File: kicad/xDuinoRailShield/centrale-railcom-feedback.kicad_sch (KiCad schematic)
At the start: 0 parts

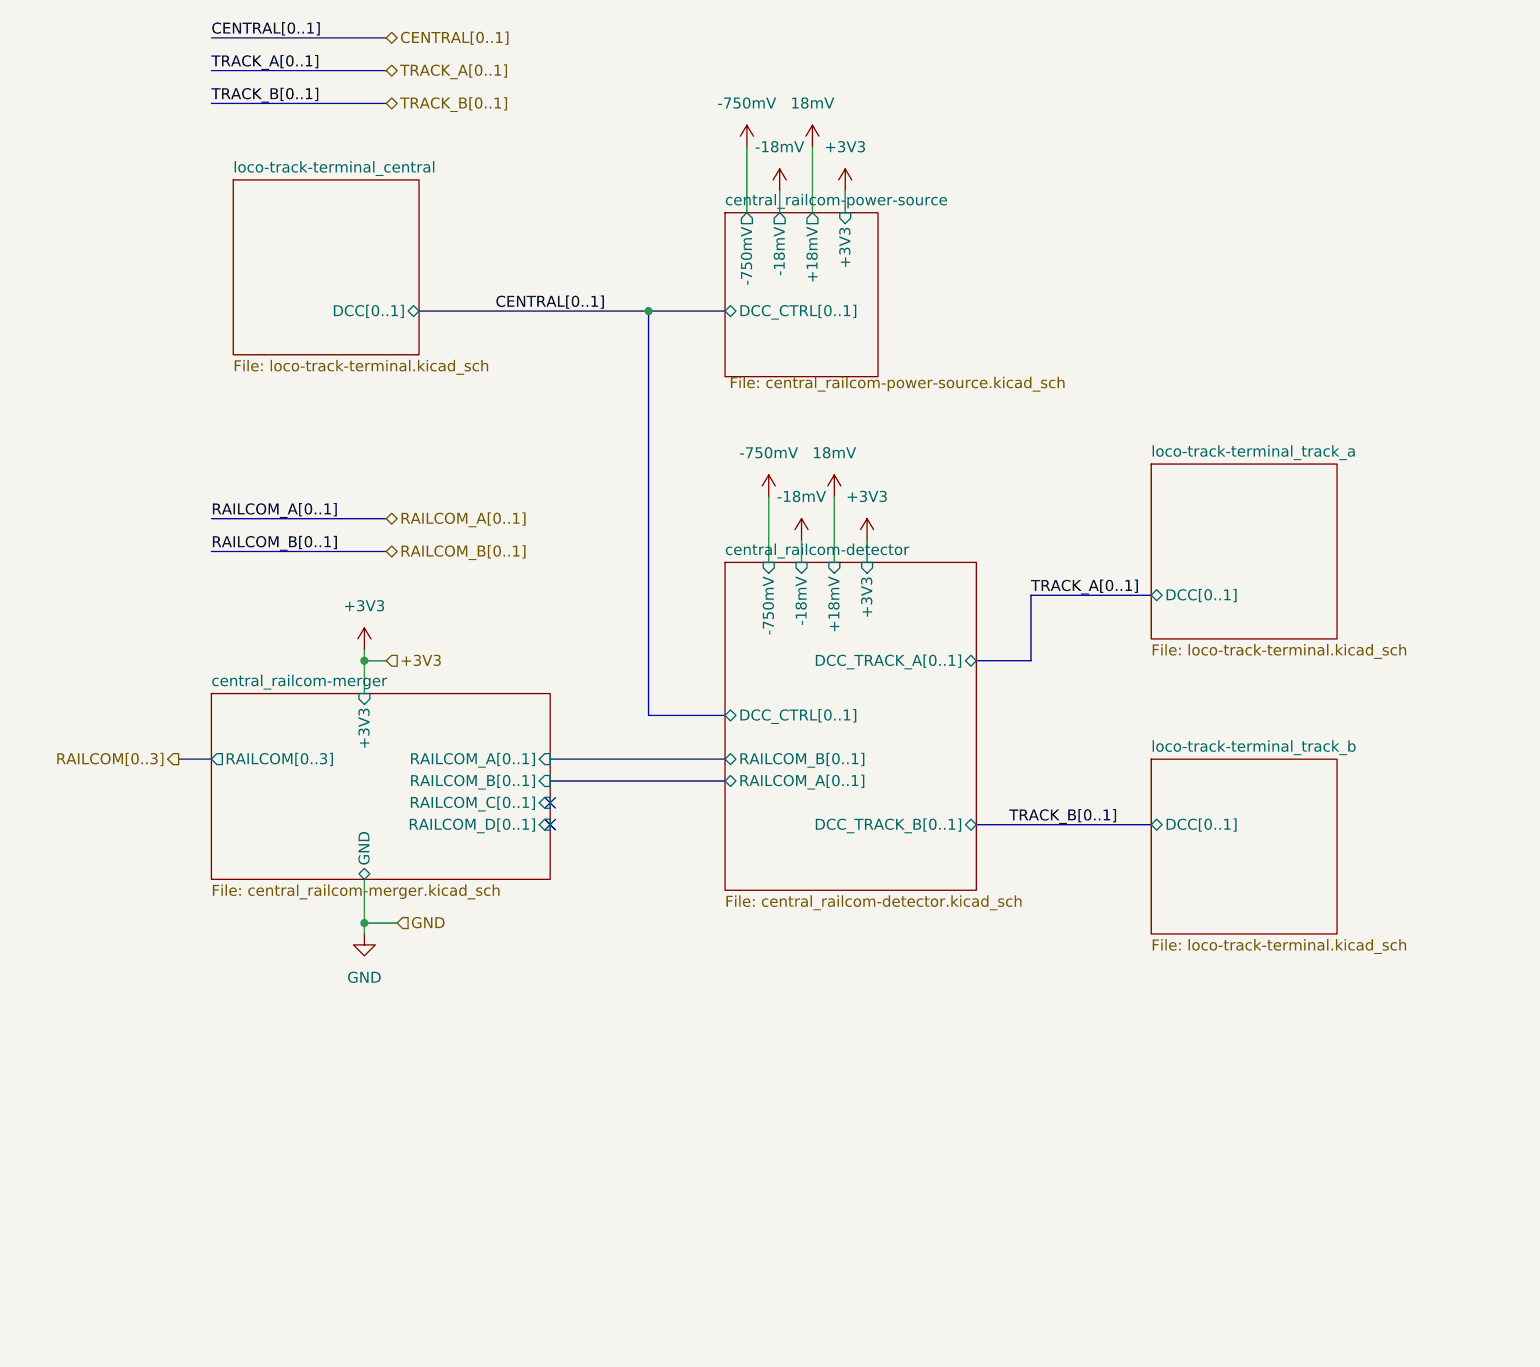
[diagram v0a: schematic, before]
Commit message: Many exiting news
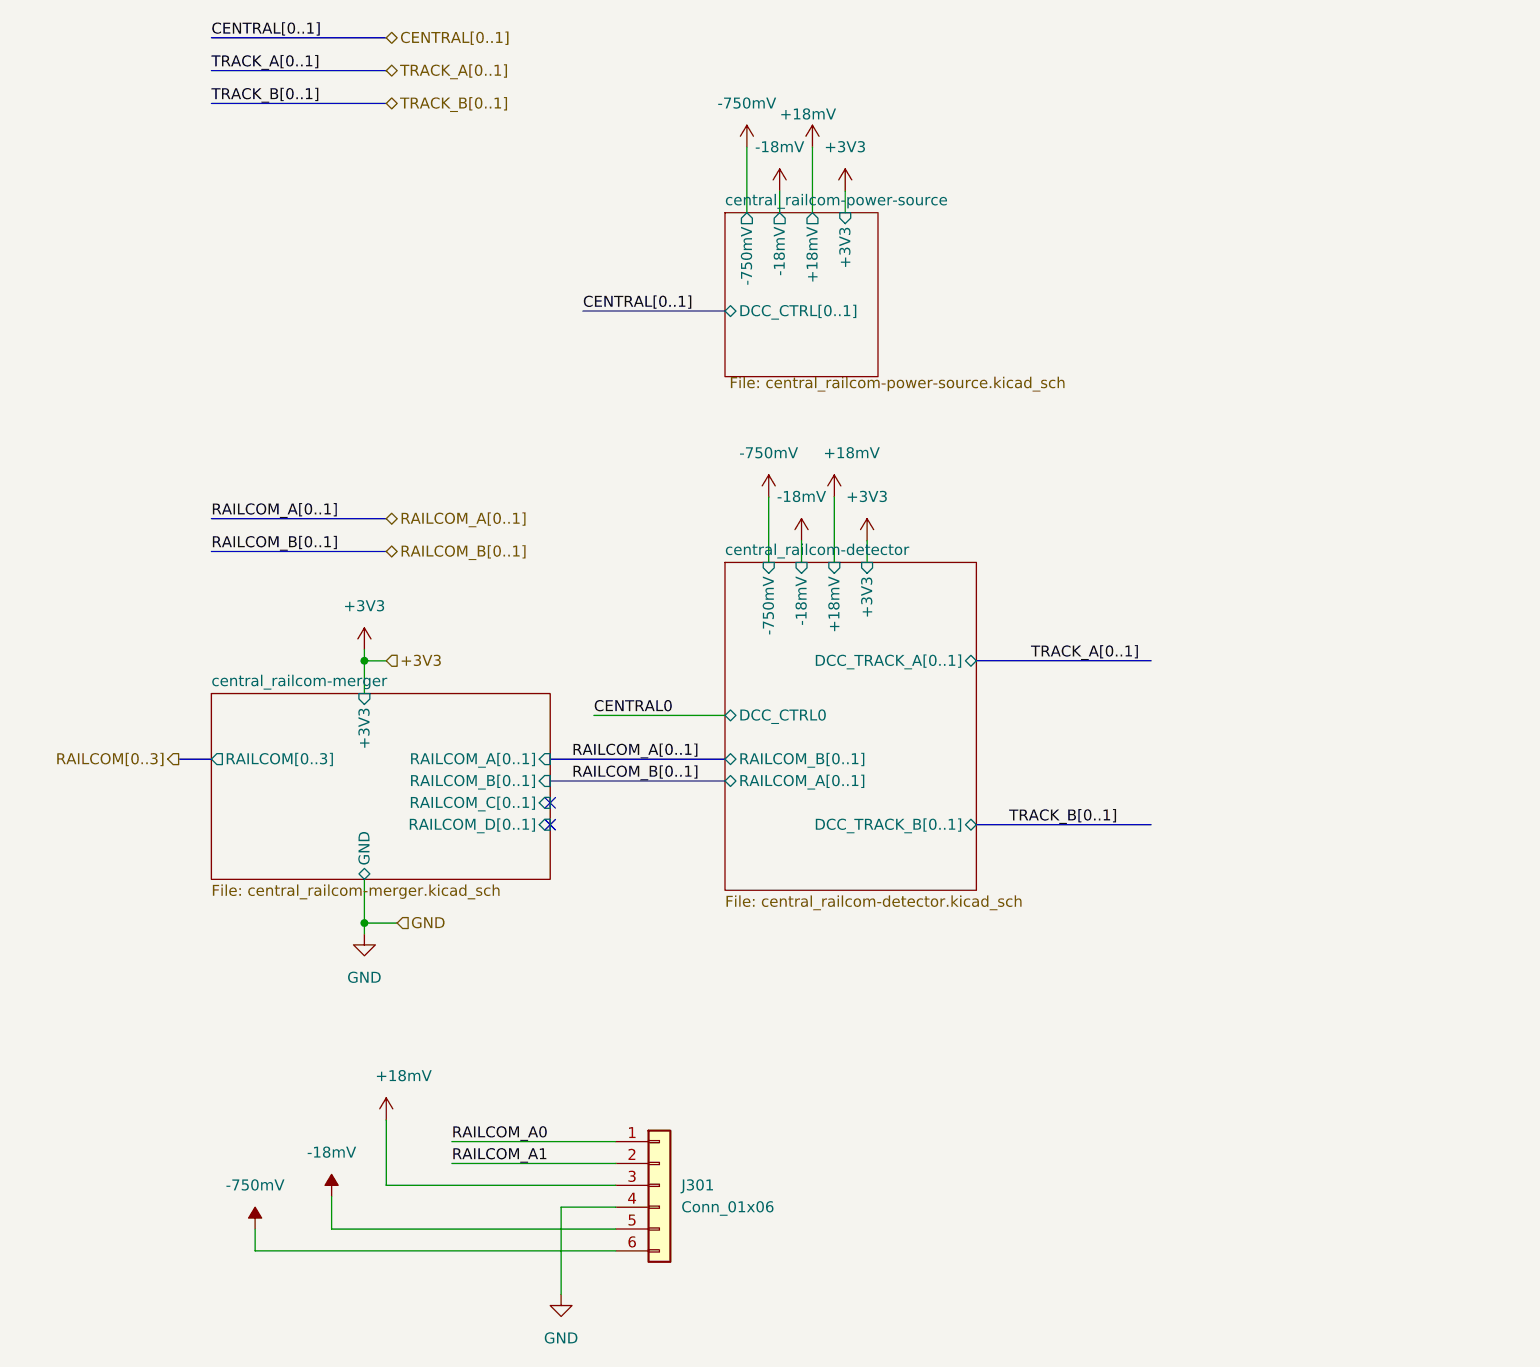
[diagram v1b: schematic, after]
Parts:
- added J301: Conn_01x06, Connector_Wire:SolderWire-0.5sqmm_1x06_P4.6mm_D0.9mm_OD2.1mm_Relief, symbol Connector_Generic:Conn_01x06
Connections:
- net -18mV: now also J301.5 (Pin_5)
- net -750mV: now also J301.6 (Pin_6)
- net GND: now also J301.4 (Pin_4)
- new net +18mV: J301.3 (Pin_3)
- new net RAILCOM_A0: J301.1 (Pin_1)
- new net RAILCOM_A1: J301.2 (Pin_2)
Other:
- removed sheet loco-track-terminal_central
- removed sheet loco-track-terminal_track_a
- removed sheet loco-track-terminal_track_b
- sheet central_railcom-detector ports: added DCC_CTRL0; removed DCC_CTRL[0..1]
